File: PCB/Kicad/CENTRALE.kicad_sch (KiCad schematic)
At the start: 75 parts, among them IC2 LM358D, J2 RJ11, J3 RJ11, P1 PINHD-1X4, P2 PINHD-1X4, U1 MCP2562-E{slash}SN

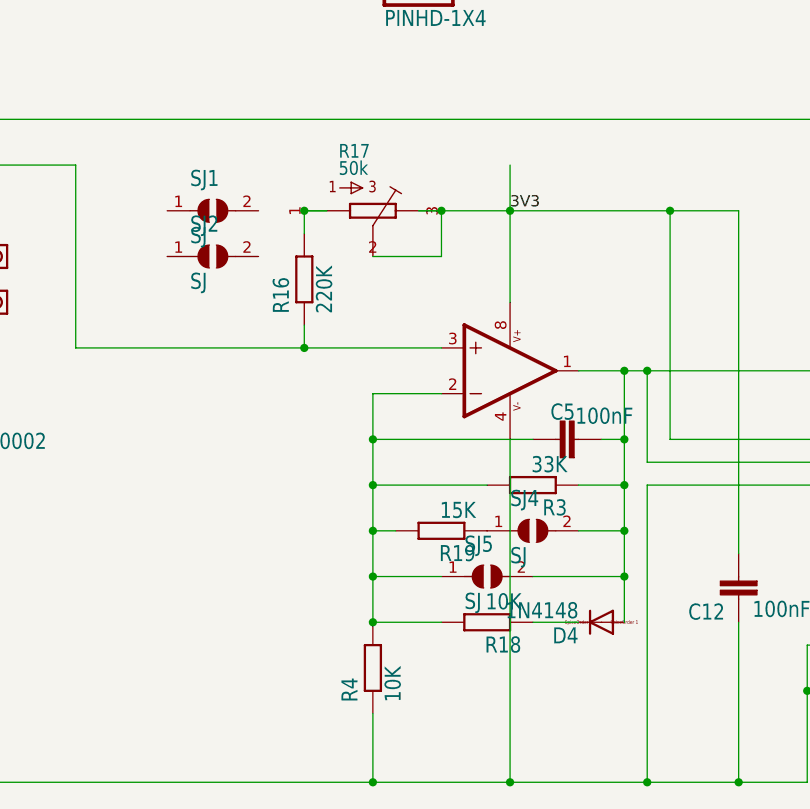
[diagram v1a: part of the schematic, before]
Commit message: PCB c3
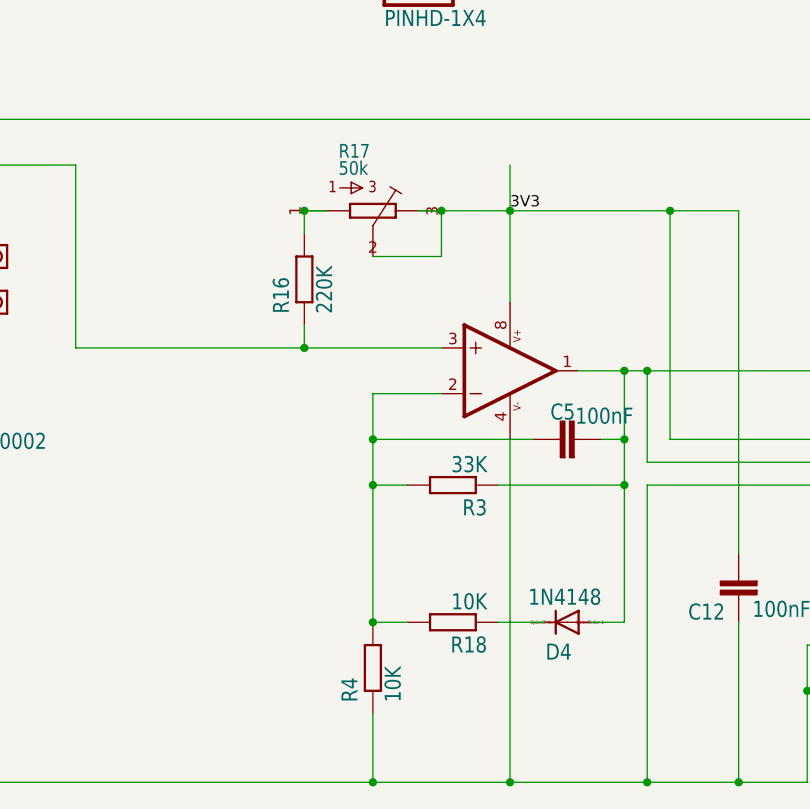
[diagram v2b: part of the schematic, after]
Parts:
- removed R19: 15K, R0805, symbol CENTRALE02c3-eagle-import:R-EU_R0805
- removed SJ1, SJ2, SJ4, SJ5: SJ, SJ, symbol CENTRALE02c3-eagle-import:SJ
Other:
- moved on the sheet: D4, R18, R3

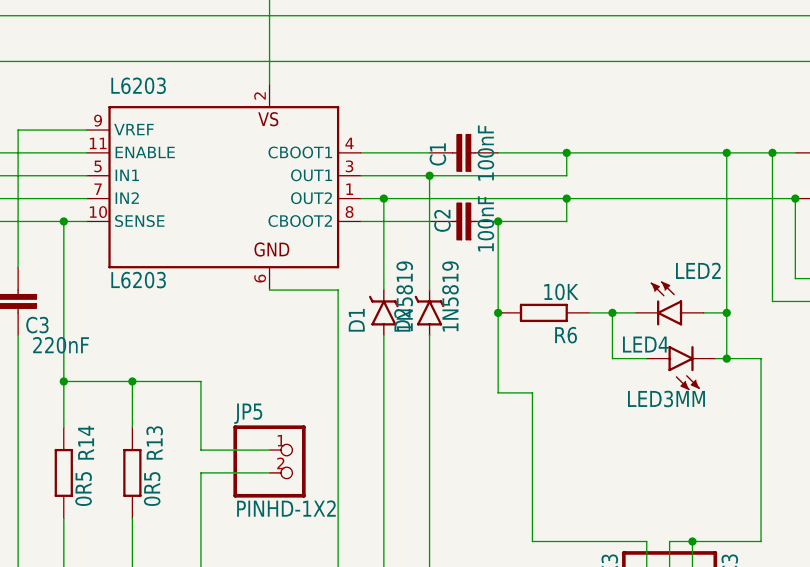
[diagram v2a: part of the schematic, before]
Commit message: PCB 03c4
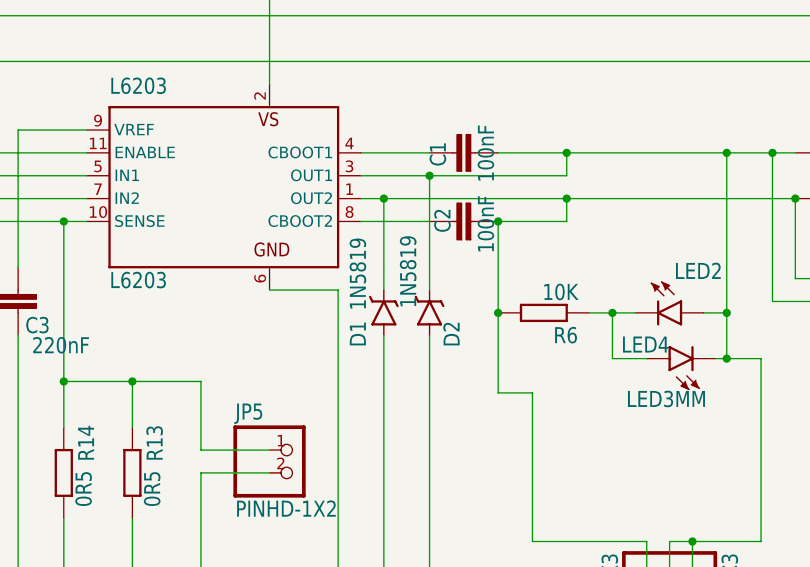
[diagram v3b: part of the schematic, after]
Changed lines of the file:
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@@
 		(dnp no)
 		(property "Reference" "D1"
-			(at 203.835 225.806 0)
+			(at 203.962 227.33 0)
 			(effects
 				(font
@@
 		)
 		(property "Value" "1N5819"
-			(at 209.169 225.806 0)
+			(at 203.962 223.266 0)
 			(effects
 				(font
@@
 		(dnp no)
 		(property "Reference" "D2"
-			(at 208.915 225.806 0)
+			(at 214.376 227.33 0)
 			(effects
 				(font
@@
 		)
 		(property "Value" "1N5819"
-			(at 214.249 225.806 0)
-			(effects
-				(font
+			(at 209.55 223.012 0)
+			(effects
+				(font
